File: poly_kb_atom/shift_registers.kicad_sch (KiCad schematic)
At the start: 5 parts

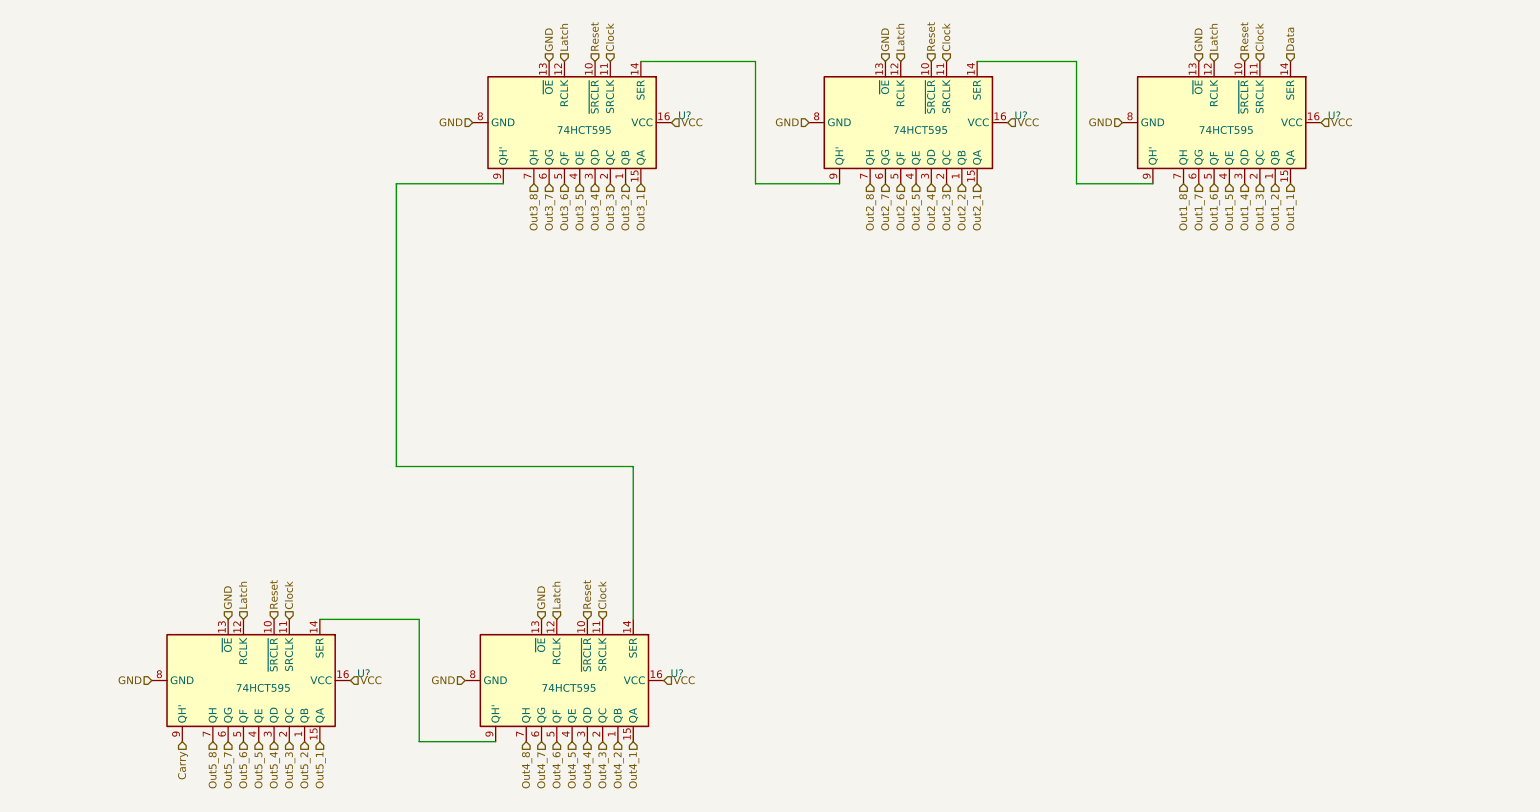
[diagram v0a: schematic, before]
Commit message: split kb prototype, left side
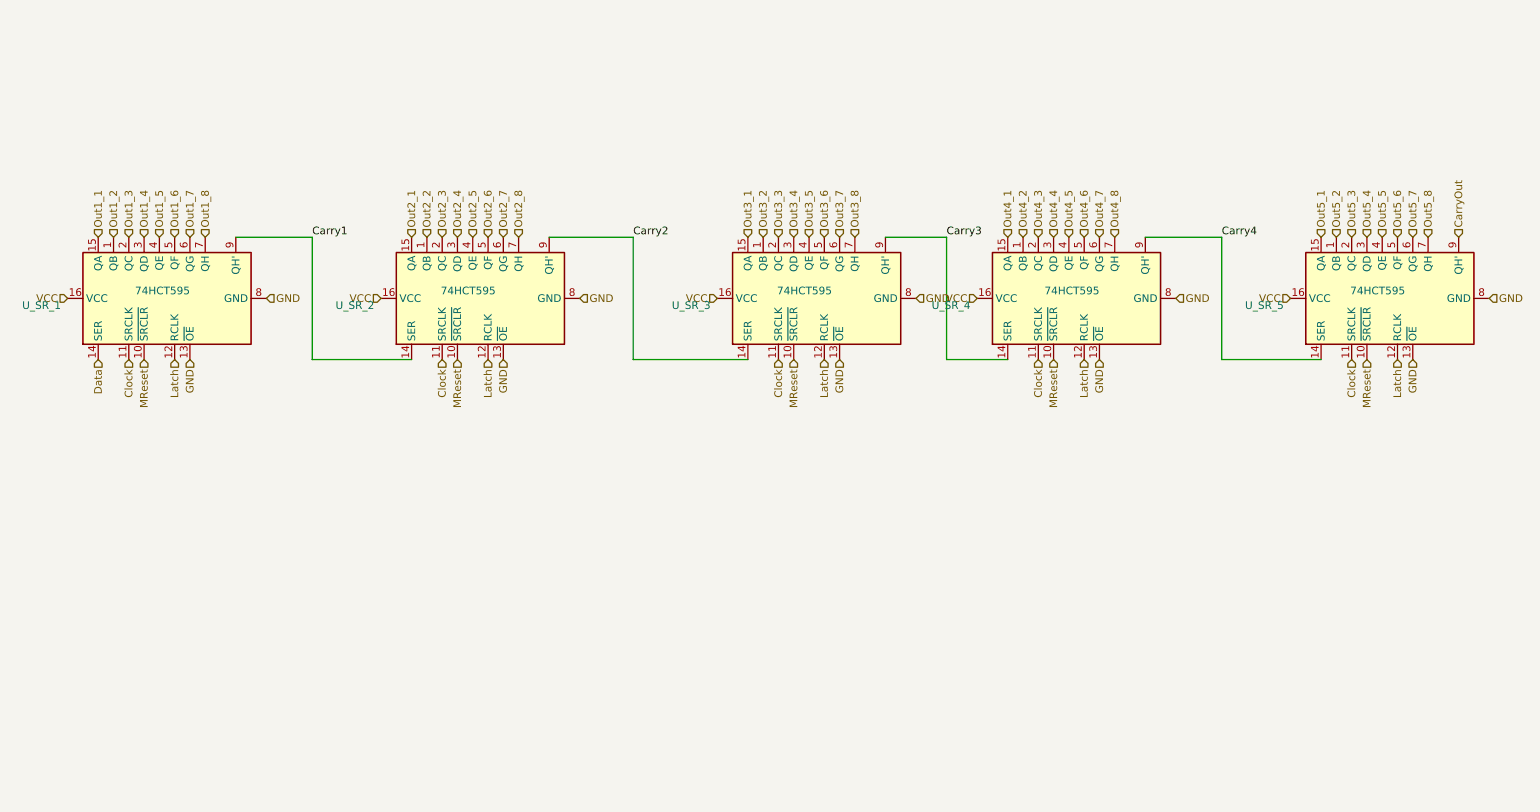
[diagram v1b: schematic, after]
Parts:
- gave numbers to parts that had none: 5
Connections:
- net Carry4: now reaches U_SR_4.9 (QH'), U_SR_5.14 (SER)
- net Carry2: now reaches U_SR_2.9 (QH'), U_SR_3.14 (SER)
- net Carry3: now reaches U_SR_3.9 (QH'), U_SR_4.14 (SER)
- net Carry1: now reaches U_SR_1.9 (QH'), U_SR_2.14 (SER)
- net Carry renamed CarryOut
- net Reset renamed MReset
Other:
- moved on the sheet: U_SR_1, U_SR_2, U_SR_3, U_SR_4, U_SR_5
